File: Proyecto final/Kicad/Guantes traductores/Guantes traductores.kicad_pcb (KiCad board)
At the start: 4 copper layers, 66.7 x 54.2 mm, 100 parts, among them J1 USB_C_Receptacle_USB2.0_16P, J10 Contacto1, J11 Contacto2, J12 Contacto3, J13 Contacto4, J3 Flex1, J4 Flex2, J5 Flex3, J6 Flex4, J7 Flex5, SW1 SW_SPST, SW2 SW_SPST, U1 ESP32-C3-WROOM-02, U10 TPS63020DSJR, U2 ADS7128IRTER, U3 USBLC6-2SC6, U4 LMV324, U5 LMV324, U6 SS12D10G5, U7 TP4056 Board, U8 BNO055, U9 HSMF-C113_C6795902

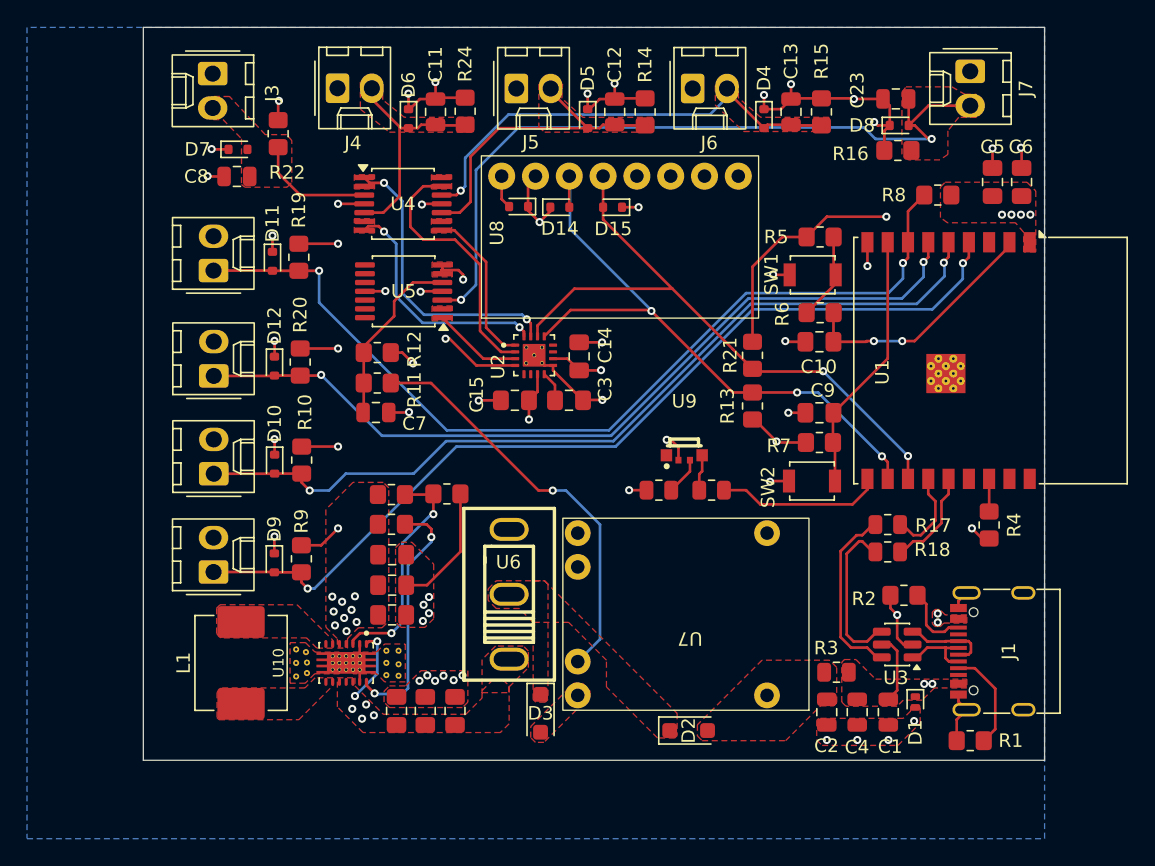
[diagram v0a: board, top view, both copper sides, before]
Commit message: Ajustes y mounting holes
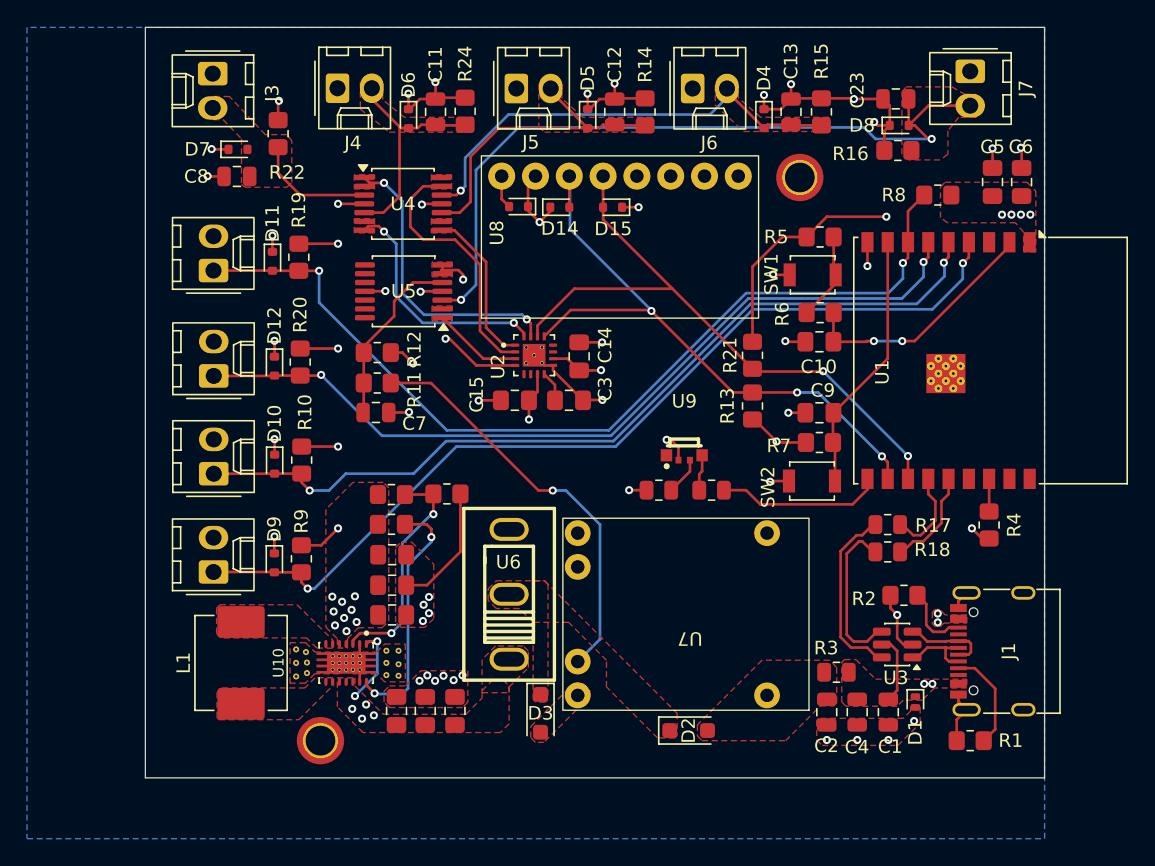
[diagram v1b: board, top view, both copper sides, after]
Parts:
- added H1: MountingHole_2.2mm_M2_ISO7380_Pad_TopOnly, MountingHole:MountingHole_2.2mm_M2_ISO7380_Pad_TopOnly, F.Cu at (154.9, 138.3)
- added H2: MountingHole_2.2mm_M2_ISO7380_Pad_TopOnly, MountingHole:MountingHole_2.2mm_M2_ISO7380_Pad_TopOnly, F.Cu at (119.5, 180.0)
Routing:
- net +3.3V: track 85.6 -> 57.0 mm
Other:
- board size 66.7 x 54.2 mm -> 66.5 x 55.5 mm
